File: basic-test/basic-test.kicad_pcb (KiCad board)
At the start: 2 copper layers, 37 x 63 mm, 45 parts, among them J1 RAPC722X, Q1 AO3400A, U1 A000053

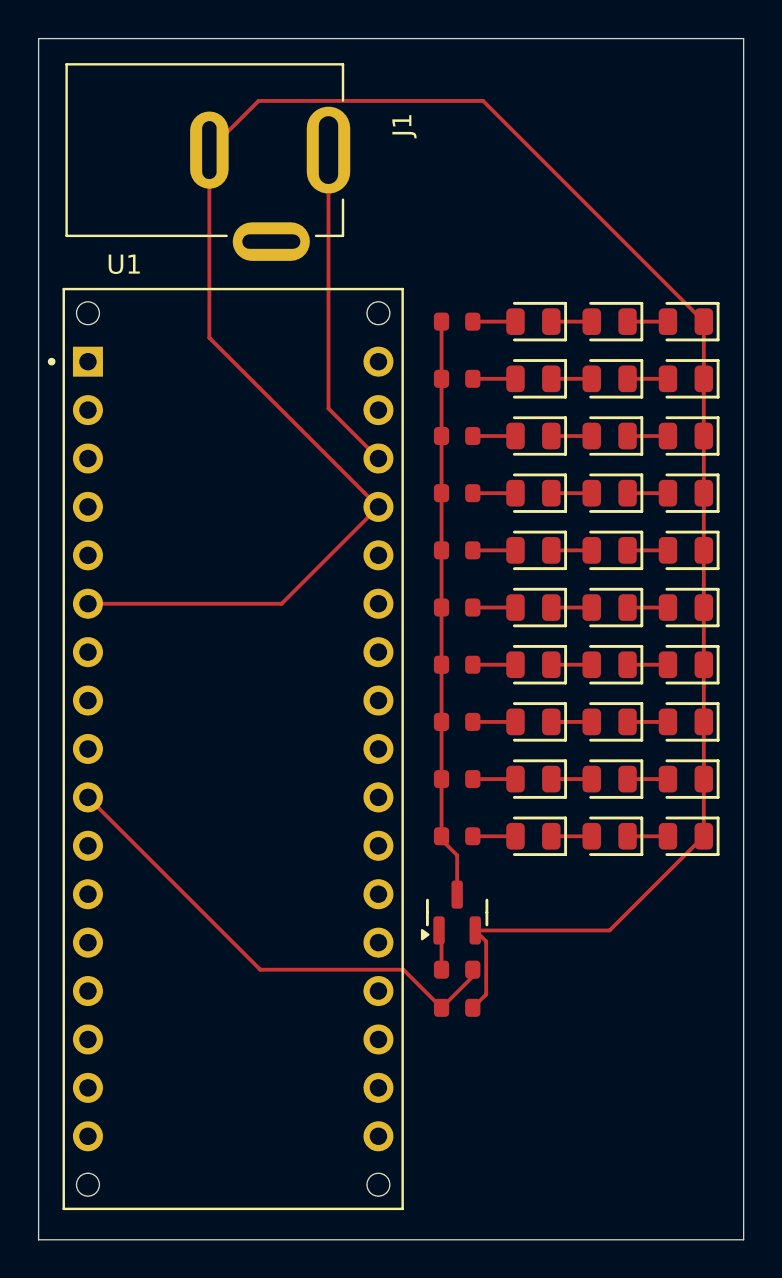
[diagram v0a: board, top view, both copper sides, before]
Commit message: fix ciruit
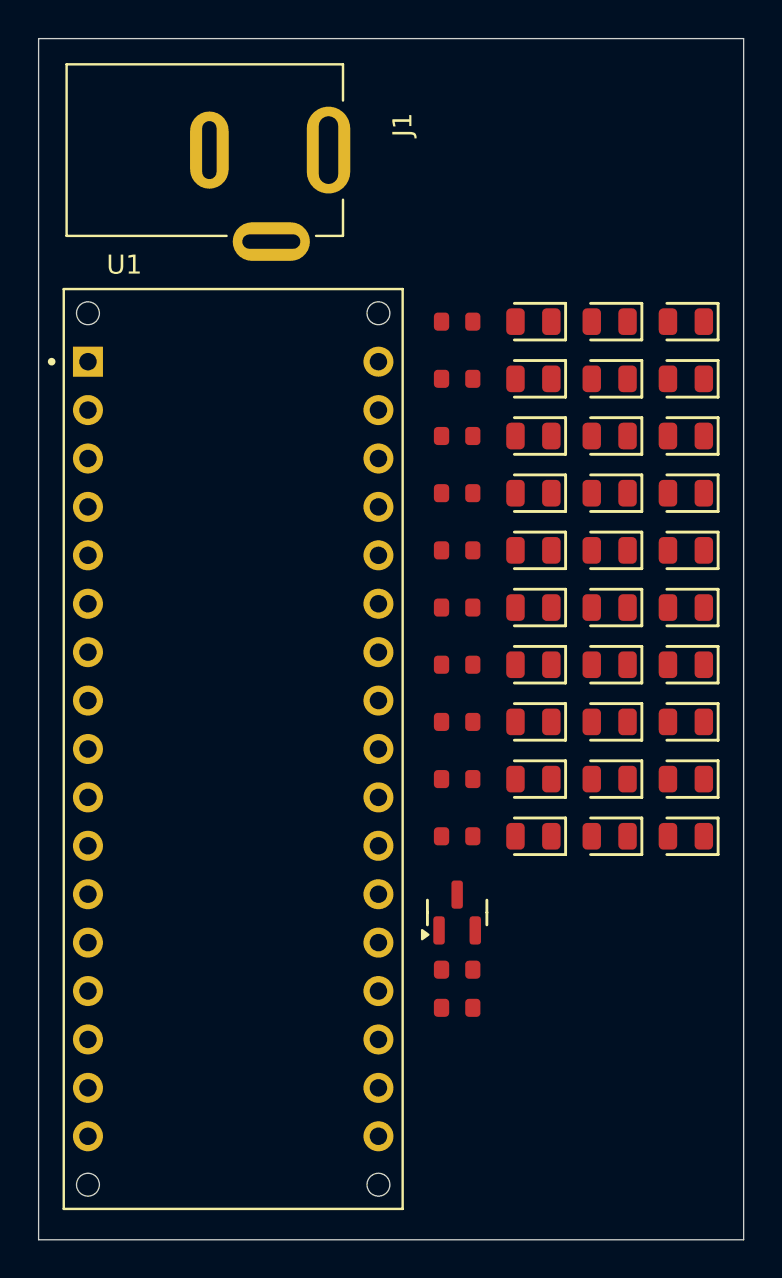
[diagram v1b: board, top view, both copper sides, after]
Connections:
- D12 pad 1: GND -> Net-(Q1-D)
- D15 pad 1: GND -> Net-(Q1-D)
- D18 pad 1: GND -> Net-(Q1-D)
- D21 pad 1: GND -> Net-(Q1-D)
- D24 pad 1: GND -> Net-(Q1-D)
- D27 pad 1: GND -> Net-(Q1-D)
- D3 pad 1: GND -> Net-(Q1-D)
- D30 pad 1: GND -> Net-(Q1-D)
- D6 pad 1: GND -> Net-(Q1-D)
- D9 pad 1: GND -> Net-(Q1-D)
- R1 pad 1: Net-(Q1-D) -> +7.5V
- R10 pad 1: Net-(Q1-D) -> +7.5V
- R2 pad 1: Net-(Q1-D) -> +7.5V
- R3 pad 1: Net-(Q1-D) -> +7.5V
- R4 pad 1: Net-(Q1-D) -> +7.5V
- R5 pad 1: Net-(Q1-D) -> +7.5V
- R6 pad 1: Net-(Q1-D) -> +7.5V
- R7 pad 1: Net-(Q1-D) -> +7.5V
- R8 pad 1: Net-(Q1-D) -> +7.5V
- R9 pad 1: Net-(Q1-D) -> +7.5V
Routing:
- net GND: track 117.2 -> 0.00 mm
- net Net-(Q1-D): track 30.4 -> 0.00 mm
- net Net-(U1-5(PWM)): track 25.8 -> 0.00 mm
- net +7.5V: track 17.3 -> 0.00 mm
- net Net-(D7-Pad2): track 2.24 -> 0.00 mm
- net Net-(D4-Pad2): track 2.24 -> 0.00 mm
- net Net-(D28-Pad2): track 2.24 -> 0.00 mm
- net Net-(D25-Pad2): track 2.24 -> 0.00 mm
- net Net-(D22-Pad2): track 2.24 -> 0.00 mm
- net Net-(D19-Pad2): track 2.24 -> 0.00 mm
- net Net-(D16-Pad2): track 2.24 -> 0.00 mm
- net Net-(D13-Pad2): track 2.24 -> 0.00 mm
- net Net-(D10-Pad2): track 2.24 -> 0.00 mm
- net Net-(D1-Pad2): track 2.24 -> 0.00 mm
- net Net-(D8-Pad1): track 2.12 -> 0.00 mm
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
